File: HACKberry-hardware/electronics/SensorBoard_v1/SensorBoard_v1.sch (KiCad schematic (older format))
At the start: 4 parts, among them U1 3-CONDUCTOR_MINIATUIRE_JACK_M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, U2 TPR-105

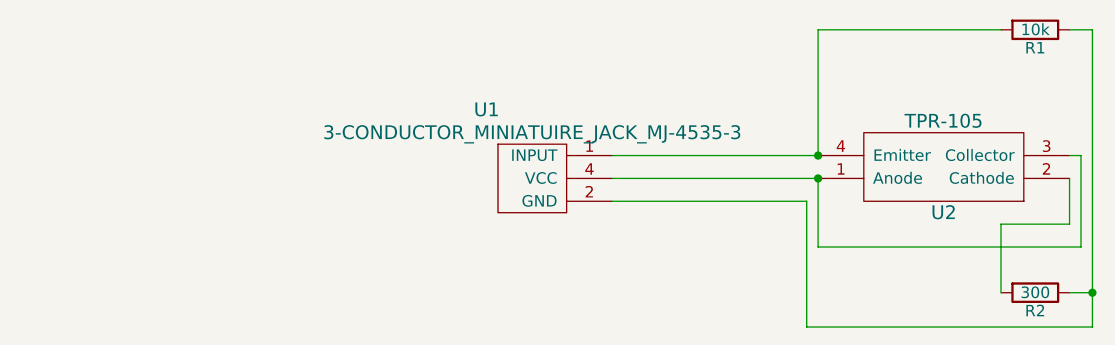
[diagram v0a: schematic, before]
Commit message: Added garber data of SensorBoard
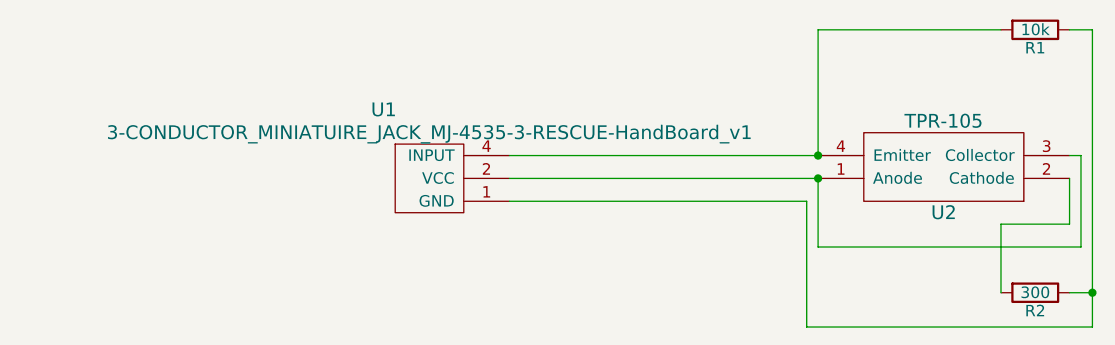
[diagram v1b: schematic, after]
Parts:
- removed U1: 3-CONDUCTOR_MINIATUIRE_JACK_MJ-4535-3, symbol 3-CONDUCTOR_MINIATUIRE_JACK_MJ-4535-3-RESCUE-SensorBoard_v1
- added U1: 3-CONDUCTOR_MINIATUIRE_JACK_MJ-4535-3-RESCUE-Hand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, HACKberry_v1:MINIATURE_JACK_MJ-4535-3, symbol 3-CONDUCTOR_MINIATUIRE_JACK_MJ-4535-3-RESCUE-HandBoard_v1
- R1, R2: footprint (none) -> Resistors_SMD:R_0603_HandSoldering
- U2: footprint (none) -> HACKberry_v1:TPR-105smd
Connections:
- net at R1.2, U2.4 (Emitter): now also U1.4 (INPUT)
- net at R1.1, R2.1: now also U1.1 (GND)
- net at U2.1 (Anode), U2.3 (Collector): now also U1.2 (VCC)
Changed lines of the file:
@@
 LIBS:myParts
 LIBS:SensorBoard_v1-cache
+LIBS:HACKberry_v1
 EELAYER 25 0
 EELAYER END
@@
 $EndDescr
 $Comp
-L 3-CONDUCTOR_MINIATUIRE_JACK_MJ-4535-3-RESCUE-SensorBoard_v1 U1
-U 1 1 55601F64
-P 4750 4000
-F 0 "U1" H 4550 4300 60  0000 C CNN
-F 1 "3-CONDUCTOR_MINIATUIRE_JACK_MJ-4535-3" H 4750 4200 60  0000 C CNN
-F 2 "" H 4750 4200 60  0000 C CNN
-F 3 "" H 4750 4200 60  0000 C CNN
-	1    4750 4000
-	1    0    0    -1
-$EndComp
-$Comp
 L TPR-105 U2
 U 1 1 55602C89
@@
 F 0 "U2" H 6550 4150 60  0000 C CNN
 F 1 "TPR-105" H 6550 3750 60  0000 C CNN
-F 2 "" H 6550 3950 60  0000 C CNN
+F 2 "HACKberry_v1:TPR-105smd" H 6550 3950 60  0001 C CNN
 F 3 "" H 6550 3950 60  0000 C CNN
 	1    6550 3950
@@
 F 0 "R1" V 7030 3350 50  0000 C CNN
 F 1 "10k" V 6950 3350 50  0000 C CNN
-F 2 "" V 6880 3350 30  0000 C CNN
+F 2 "Resistors_SMD:R_0603_HandSoldering" V 6880 3350 30  0001 C CNN
 F 3 "" H 6950 3350 30  0000 C CNN
 	1    6950 3350
@@
 F 0 "R2" V 7030 4500 50  0000 C CNN
 F 1 "300" V 6950 4500 50  0000 C CNN
-F 2 "" V 6880 4500 30  0000 C CNN
+F 2 "Resistors_SMD:R_0603_HandSoldering" V 6880 4500 30  0001 C CNN
 F 3 "" H 6950 4500 30  0000 C CNN
 	1    6950 4500
@@
 $EndComp
 Wire Wire Line
-	5100 3900 6000 3900
+	4650 3900 6000 3900
 Wire Wire Line
 	6800 3350 6000 3350
@@
 	6000 3350 6000 3900
 Wire Wire Line
-	5100 4000 6000 4000
+	4650 4000 6000 4000
 Wire Wire Line
 	7100 4000 7100 4200
@@
 	6000 4300 6000 4000
 Wire Wire Line
-	5100 4100 5950 4100
+	4650 4100 5950 4100
 Wire Wire Line
 	5950 4100 5950 4650
 Wire Wire Line
-	5950 4650 7200 4650
+	7200 4650 5950 4650
 Connection ~ 7200 4500
 Wire Wire Line
-	7200 4650 7200 3350
+	7200 3350 7200 4650
 Wire Wire Line
 	7150 3900 7150 4300
 Connection ~ 6000 3900
 Connection ~ 6000 4000
+$Comp
+L 3-CONDUCTOR_MINIATUIRE_JACK_MJ-4535-3-RESCUE-HandBoard_v1 U1
+U 1 1 55C4B6D8
+P 4300 4000
+F 0 "U1" H 4100 4300 60  0000 C CNN
+F 1 "3-CONDUCTOR_MINIATUIRE_JACK_MJ-4535-3-RESCUE-HandBoard_v1" H 4300 4200 60  0000 C CNN
+F 2 "HACKberry_v1:MINIATURE_JACK_MJ-4535-3" H 4300 4200 60  0001 C CNN
+F 3 "" H 4300 4200 60  0000 C CNN
+	1    4300 4000
+	1    0    0    -1
+$EndComp
 $EndSCHEMATC
